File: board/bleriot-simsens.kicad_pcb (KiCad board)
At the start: 2 copper layers, 40 x 42 mm, 24 parts, among them J3 POWER, J4 RS485, U1 LM1117MP-3.3, U4 MAX485E, U5 PAN2110P0AA, U6 PY32F030F1xPx, X2 SWD, Y2 16MHz

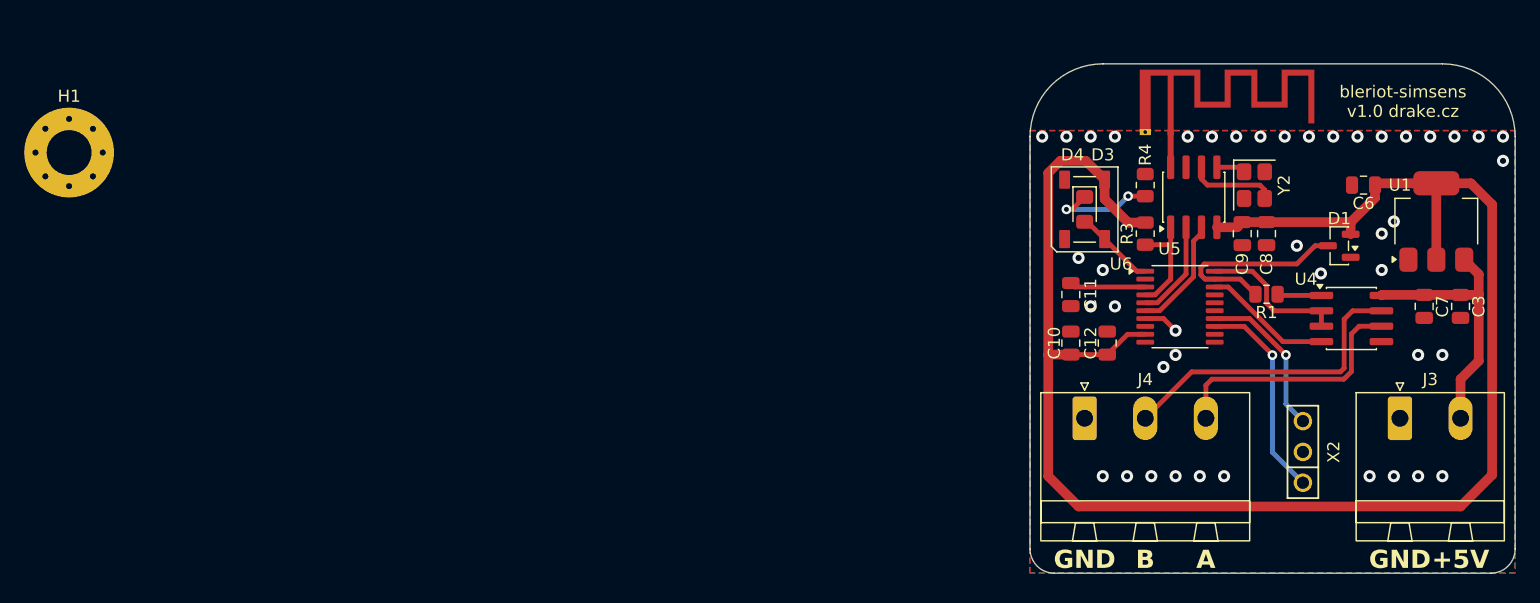
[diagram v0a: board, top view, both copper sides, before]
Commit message: WIP
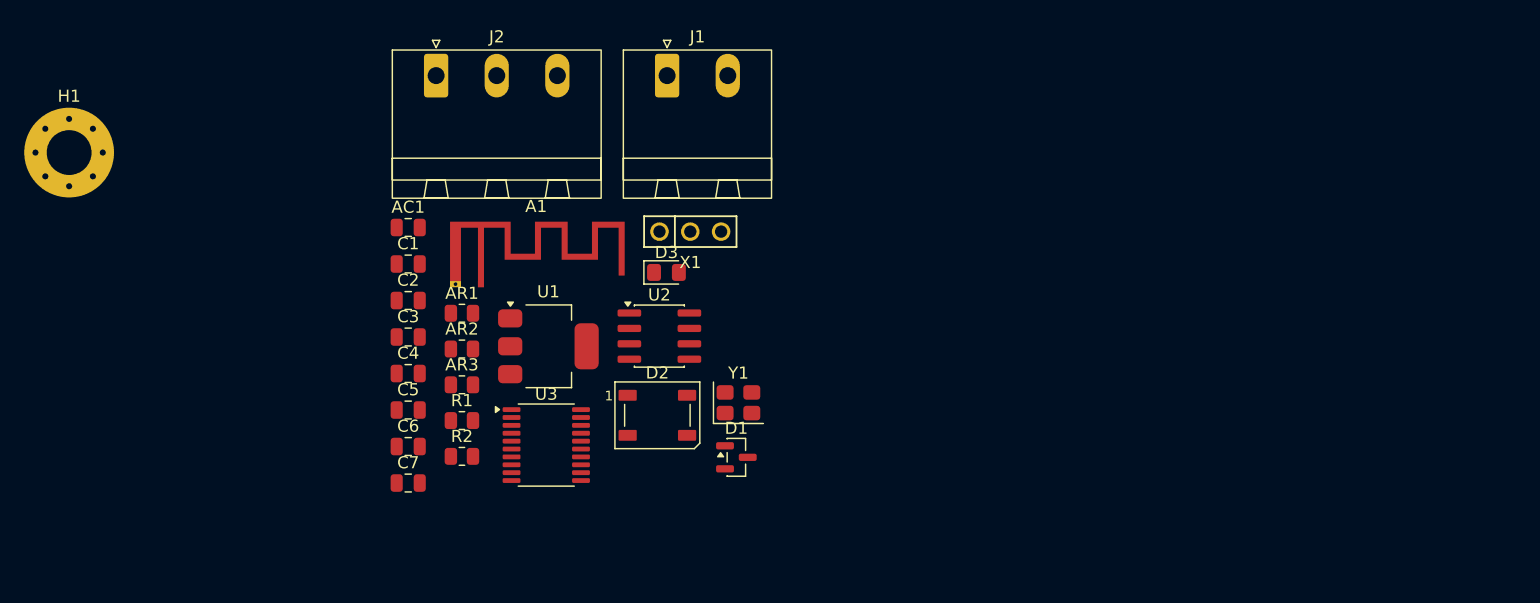
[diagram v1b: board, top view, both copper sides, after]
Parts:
- removed A2: Antenna_Shield, RF_Antenna:Texas_SWRA117D_2.4GHz_Right
- removed C10, C8: 1u, Capacitor_SMD:C_0805_2012Metric
- removed C11, C12, C9: 100n, Capacitor_SMD:C_0805_2012Metric
- removed D4: LED, LED_SMD:LED_0805_2012Metric_Pad1.15x1.40mm_HandSolder
- removed J3: POWER, Connector_Phoenix_MSTB:PhoenixContact_MSTBA_2,5_2-G_1x02_P5.00mm_Horizontal
- removed J4: RS485, Connector_Phoenix_MSTB:PhoenixContact_MSTBA_2,5_3-G_1x03_P5.00mm_Horizontal
- removed R3: 10k, Resistor_SMD:R_0805_2012Metric
- removed R4: 330R, Resistor_SMD:R_0805_2012Metric
- removed U4: MAX485E, Package_SO:SOIC-8_3.9x4.9mm_P1.27mm
- removed U5: PAN2110P0AA, Package_SO:SOIC-8_3.9x4.9mm_P1.27mm
- removed U6: PY32F030F1xPx, Package_SO:TSSOP-20_4.4x6.5mm_P0.65mm
- removed X2: SWD, Drake:SWD
- removed Y2: 16MHz, Crystal:Crystal_SMD_3225-4Pin_3.2x2.5mm
- added A1: Antenna_Shield, RF_Antenna:Texas_SWRA117D_2.4GHz_Right, F.Cu at (96.2, 49.2)
- added AC1: 100n, Capacitor_SMD:C_0805_2012Metric, F.Cu at (90.2, 44.5)
- added AR1: 10k 0.1%, Resistor_SMD:R_0805_2012Metric, F.Cu at (94.7, 51.6)
- added AR2: 4.02k 0.1%, Resistor_SMD:R_0805_2012Metric, F.Cu at (94.7, 54.5)
- added AR3: 6.49k 0.1%, Resistor_SMD:R_0805_2012Metric, F.Cu at (94.7, 57.5)
- added C1: 10u, Capacitor_SMD:C_0805_2012Metric, F.Cu at (90.2, 47.5)
- added C2: 1u, Capacitor_SMD:C_0805_2012Metric, F.Cu at (90.2, 50.5)
- added C4: 100n, Capacitor_SMD:C_0805_2012Metric, F.Cu at (90.2, 56.5)
- added C5: 100n, Capacitor_SMD:C_0805_2012Metric, F.Cu at (90.2, 59.5)
- added D2: WS2812B, LED_SMD:LED_WS2812B_PLCC4_5.0x5.0mm_P3.2mm, F.Cu at (110.8, 60.0)
- added J1: POWER, Connector_Phoenix_MSTB:PhoenixContact_MSTBA_2,5_2-G_1x02_P5.00mm_Horizontal, F.Cu at (111.6, 32.0)
- added J2: INPUT, Connector_Phoenix_MSTB:PhoenixContact_MSTBA_2,5_3-G_1x03_P5.00mm_Horizontal, F.Cu at (92.5, 32.0)
- added R2: 330R, Resistor_SMD:R_0805_2012Metric, F.Cu at (94.7, 63.4)
- added U2: PAN2110P0AA, Package_SO:SOIC-8_3.9x4.9mm_P1.27mm, F.Cu at (110.9, 53.5)
- added U3: PY32F030F1xPx, Package_SO:TSSOP-20_4.4x6.5mm_P0.65mm, F.Cu at (101.6, 62.4)
- added X1: SWD, Drake:SWD, F.Cu at (113.5, 44.8)
- added Y1: 16MHz, Crystal:Crystal_SMD_3225-4Pin_3.2x2.5mm, F.Cu at (117.5, 58.9)
- C6: value 10u -> 1u
- D3: value WS2812B -> LED; footprint LED_SMD:LED_WS2812B_PLCC4_5.0x5.0mm_P3.2mm -> LED_SMD:LED_0805_2012Metric_Pad1.15x1.40mm_HandSolder
- R1: value 1k5 -> 10k
- moved C3 86.8 mm to (90.2, 53.5), turned to 0 degrees
- moved C7 85.0 mm to (90.2, 65.6), turned to 0 degrees
- moved C6 81.7 mm to (90.2, 62.6), turned to 0 degrees
- moved U1 73.9 mm to (101.8, 54.3), turned to 0 degrees
- moved R1 67.2 mm to (94.7, 60.4)
- moved D1 52.7 mm to (117.3, 63.4), turned to 0 degrees
- moved D3 34.9 mm to (111.5, 48.2), turned to 0 degrees
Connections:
- C3 pad 1: +5V -> +3V3
- C7 pad 1: +5V -> +3V3
- D1 pad 3: /RS485_RX -> /INPUT_MCU
- D3 pad 1: +3V3 -> Net-(D3-K)
- D3 pad 2: unconnected-(D3-DOUT-Pad2) -> /LED
- R1 pad 1: /RS485_RX -> /~{RF_CS}
- R1 pad 2: Net-(U4-RO) -> +3V3
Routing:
- net +3V3: track 139.0 -> 0.00 mm
- net /RS485_B: track 25.5 -> 0.00 mm
- net +5V: track 22.3 -> 0.00 mm
- net /RS485_A: track 21.0 -> 0.00 mm
- net Net-(U6-PA11): track 17.3 -> 0.00 mm, vias 1 -> 0
- net /RS485_RX: track 17.0 -> 0.00 mm
- net Net-(U6-PA13): track 13.2 -> 0.00 mm, vias 1 -> 0
- net /RS485_TXEN: track 12.3 -> 0.00 mm
- net /RS485_TX: track 10.7 -> 0.00 mm
- net /RF_DATA: track 9.49 -> 0.00 mm
- net /~{RF_CS}: track 9.04 -> 0.00 mm
- net Net-(D4-K): track 9.00 -> 0.00 mm, vias 2 -> 0
- net /RF_SCK: track 8.20 -> 0.00 mm
- net Net-(U5-XC0): track 7.26 -> 0.00 mm
- net /LED: track 6.69 -> 0.00 mm
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- removed copper zone on B.Cu, net GND
- removed copper zone on F.Cu, net GND
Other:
- board outline removed
- board text removed: "+5V"
- board text removed: "A"
- board text removed: "B"
- board text removed: "GND"
- board text removed: "bleriot-simsens v1.0 drake.cz"
